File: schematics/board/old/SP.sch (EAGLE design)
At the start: 24 parts

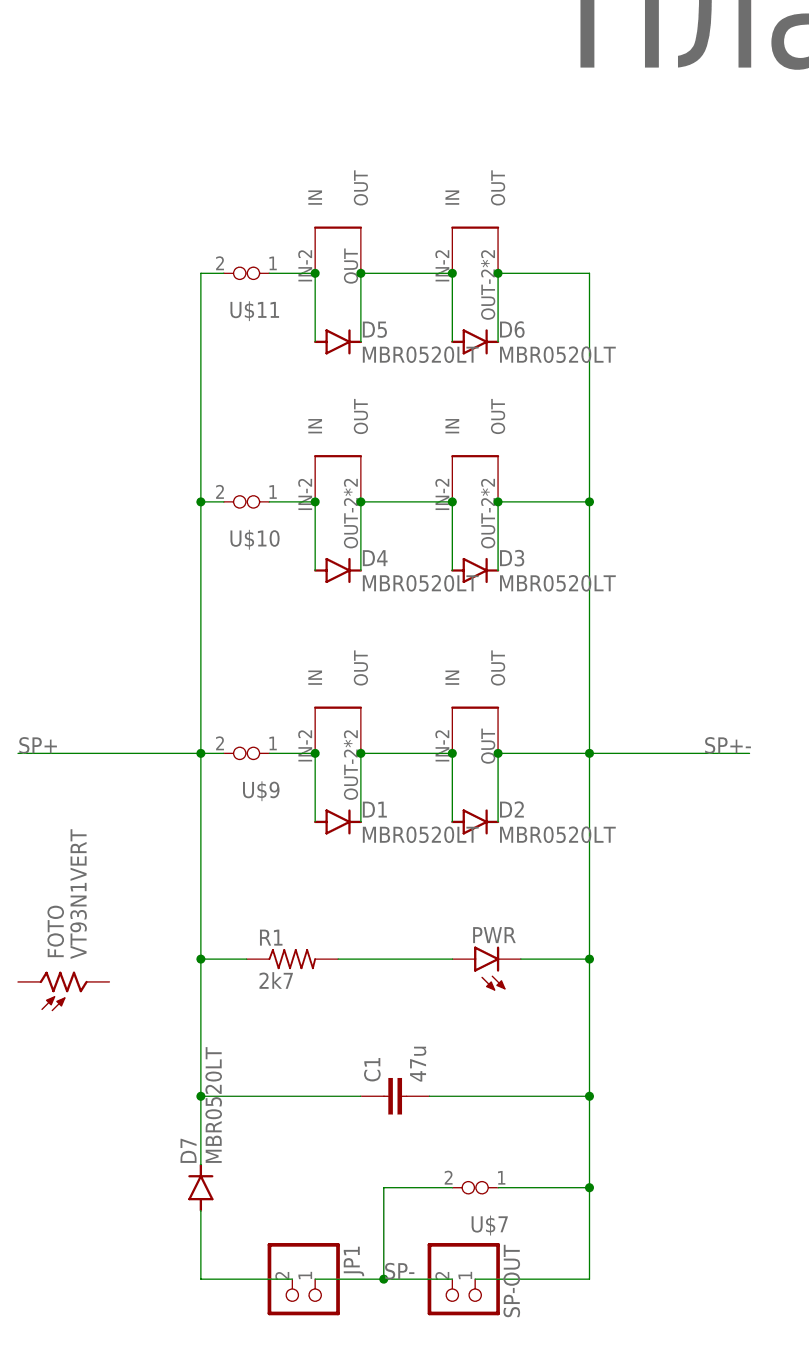
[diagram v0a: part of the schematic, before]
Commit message: Платы готовы
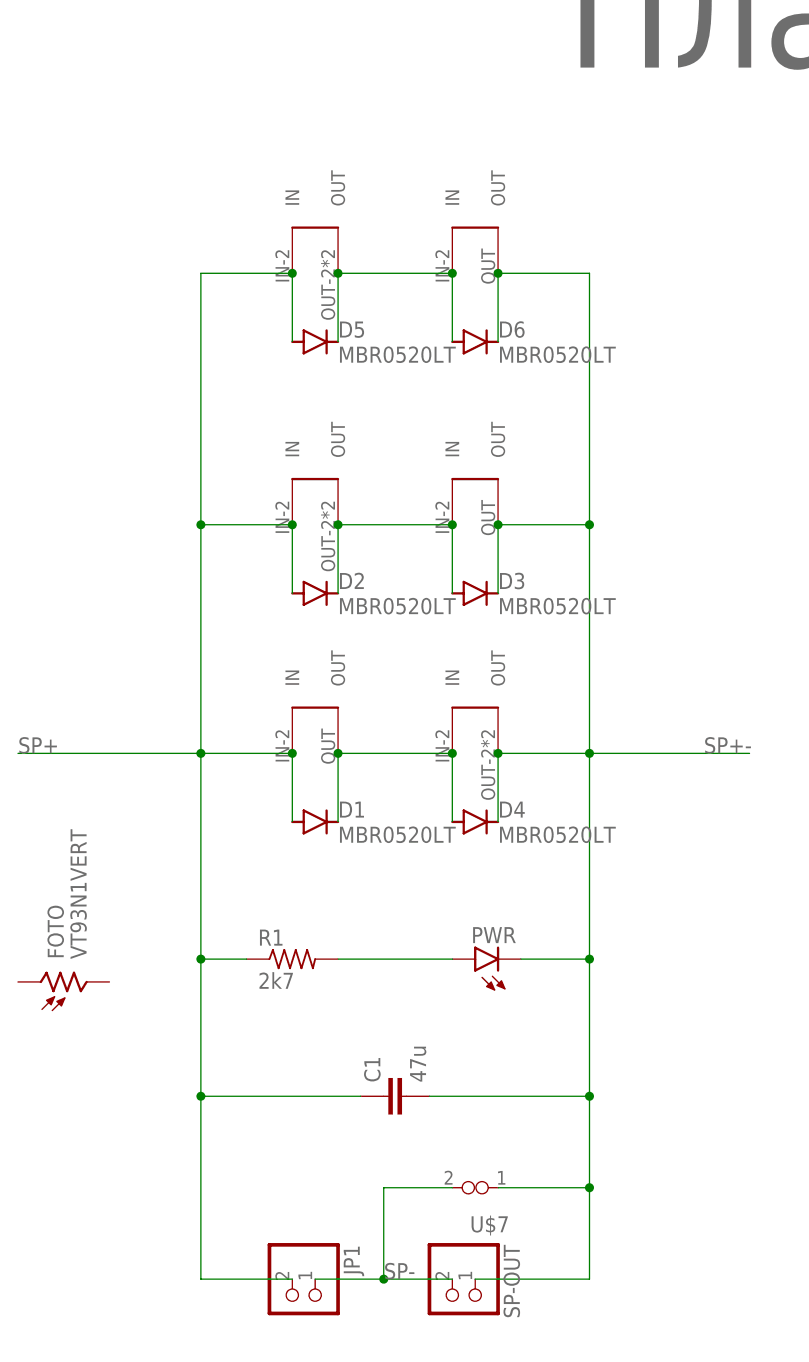
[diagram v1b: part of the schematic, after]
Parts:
- removed D7: MBR0520LT, diode:MBR0520LT
- removed U$10, U$11, U$9: (no value), KNPN-2023:VIAS-CONNECT
- U$1, U$3, U$8: value SOLAR-2_INVERT0-2 -> SOLAR-2_1; device KNPN-2023:SOLAR-2_INVERT0-2 -> KNPN-2023:SOLAR-2_1
- U$2, U$6: value SOLAR-2_INVERT1-2 -> SOLAR-2_0; device KNPN-2023:SOLAR-2_INVERT1-2 -> KNPN-2023:SOLAR-2_0
- U$4: value SOLAR-2_INVERT0-2 -> SOLAR-2_0; device KNPN-2023:SOLAR-2_INVERT0-2 -> KNPN-2023:SOLAR-2_0
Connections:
- removed net N$1: D7.A, JP1.2
- removed net N$5: D1.C, D2.A, U$1.OUT, U$2.IN
- removed net N$6: D3.A, D4.C, U$3.IN, U$4.OUT
- removed net N$7: D1.A, U$1.IN, U$9.1
- net N$2: now also D2.C, D3.A, U$2.OUT, U$3.IN; no longer D5.A, U$11.1, U$6.IN
- net N$3: now also D1.C, U$1.OUT; no longer U$10.1
- net SP+: now also D1.A, D2.A, D5.A, JP1.2, U$1.IN, U$2.IN, U$6.IN; no longer D7.C, U$10.2, U$11.2, U$9.2
- net SP+-: now also D4.C, U$4.OUT; no longer D2.C, U$2.OUT
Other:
- moved on the sheet: D1, D2, D3, D4, D5
